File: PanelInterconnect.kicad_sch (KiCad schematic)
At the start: 14 parts, among them J1 Conn_01x02, J2 Conn_01x04

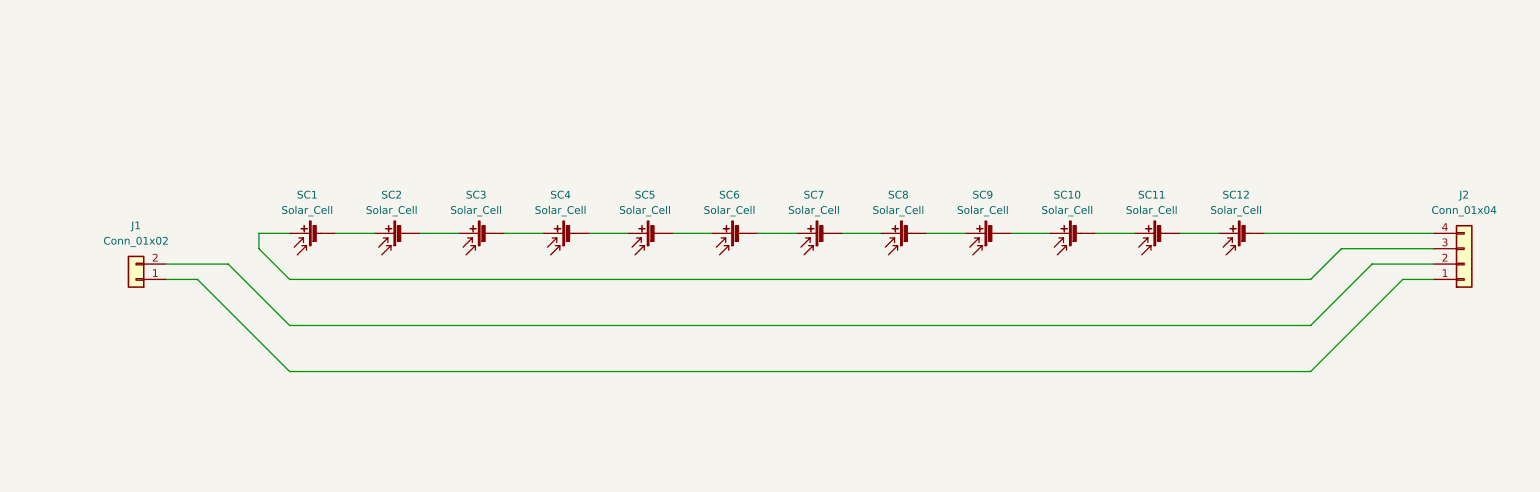
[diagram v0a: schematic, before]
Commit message: Pushing
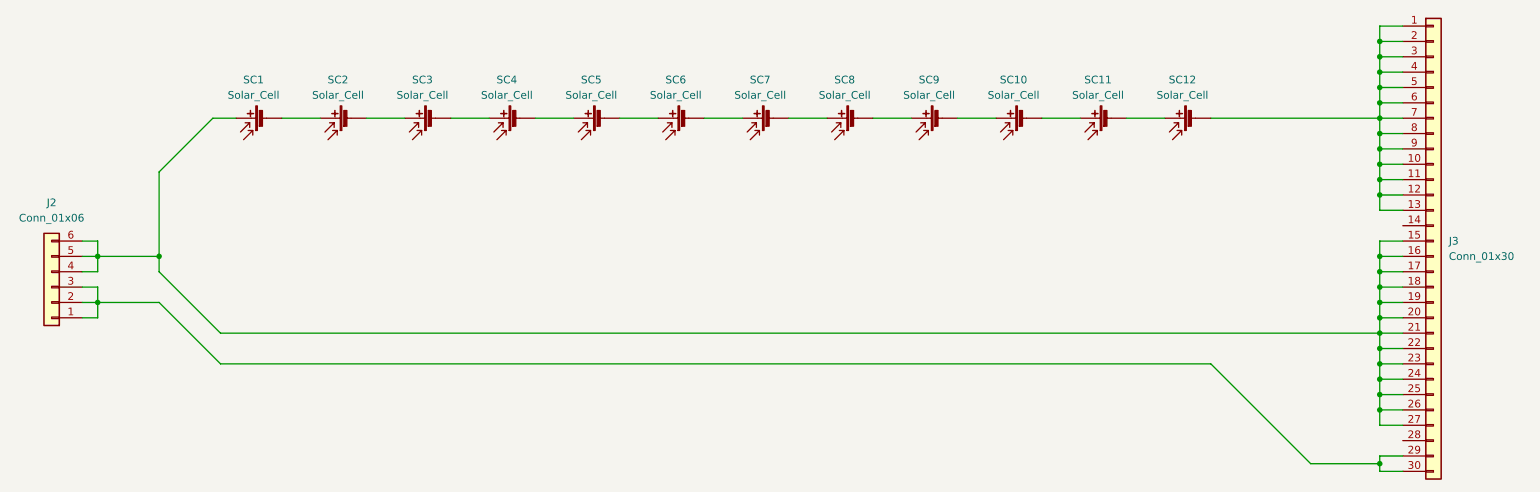
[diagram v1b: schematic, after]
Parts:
- removed J1: Conn_01x02, TerminalBlock:TerminalBlock_MaiXu_MX126-5.0-02P_1x02_P5.00mm, symbol Connector_Generic:Conn_01x02
- removed J2: Conn_01x04, TerminalBlock:TerminalBlock_MaiXu_MX126-5.0-04P_1x04_P5.00mm, symbol Connector_Generic:Conn_01x04
- added J2: Conn_01x06, Connector_FFC-FPC:Jushuo_AFC07-S06FCA-00_1x6-1MP_P0.50_Horizontal, symbol Connector_Generic:Conn_01x06
- added J3: Conn_01x30, _PanelInterconnct:FPC_30x01, symbol Connector_Generic:Conn_01x30
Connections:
- net at SC1.1 (+): now also J2.4 (Pin_4), J2.5 (Pin_5), J2.6 (Pin_6), J3.15 (Pin_15), J3.16 (Pin_16), J3.17 (Pin_17), J3.18 (Pin_18), J3.19 (Pin_19), J3.20 (Pin_20), J3.21 (Pin_21), J3.22 (Pin_22), J3.23 (Pin_23), J3.24 (Pin_24), J3.25 (Pin_25), J3.26 (Pin_26), J3.27 (Pin_27)
- net at SC12.2 (-): now also J3.1 (Pin_1), J3.10 (Pin_10), J3.11 (Pin_11), J3.12 (Pin_12), J3.13 (Pin_13), J3.2 (Pin_2), J3.3 (Pin_3), J3.4 (Pin_4), J3.5 (Pin_5), J3.6 (Pin_6), J3.7 (Pin_7), J3.8 (Pin_8), J3.9 (Pin_9)
- new net: J2.1 (Pin_1), J2.2 (Pin_2), J2.3 (Pin_3), J3.29 (Pin_29), J3.30 (Pin_30)
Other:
- moved on the sheet: SC1, SC10, SC11, SC12, SC2, SC3, SC4, SC5, SC6, SC7, SC8, SC9
